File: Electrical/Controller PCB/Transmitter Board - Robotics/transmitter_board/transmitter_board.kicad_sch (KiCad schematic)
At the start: 19 parts, among them SW1 Enable, SW2 Power, SW3 E Stop, U1 AP63203WU, U2 ESP32-S3-ZERO, U3 COM-09032

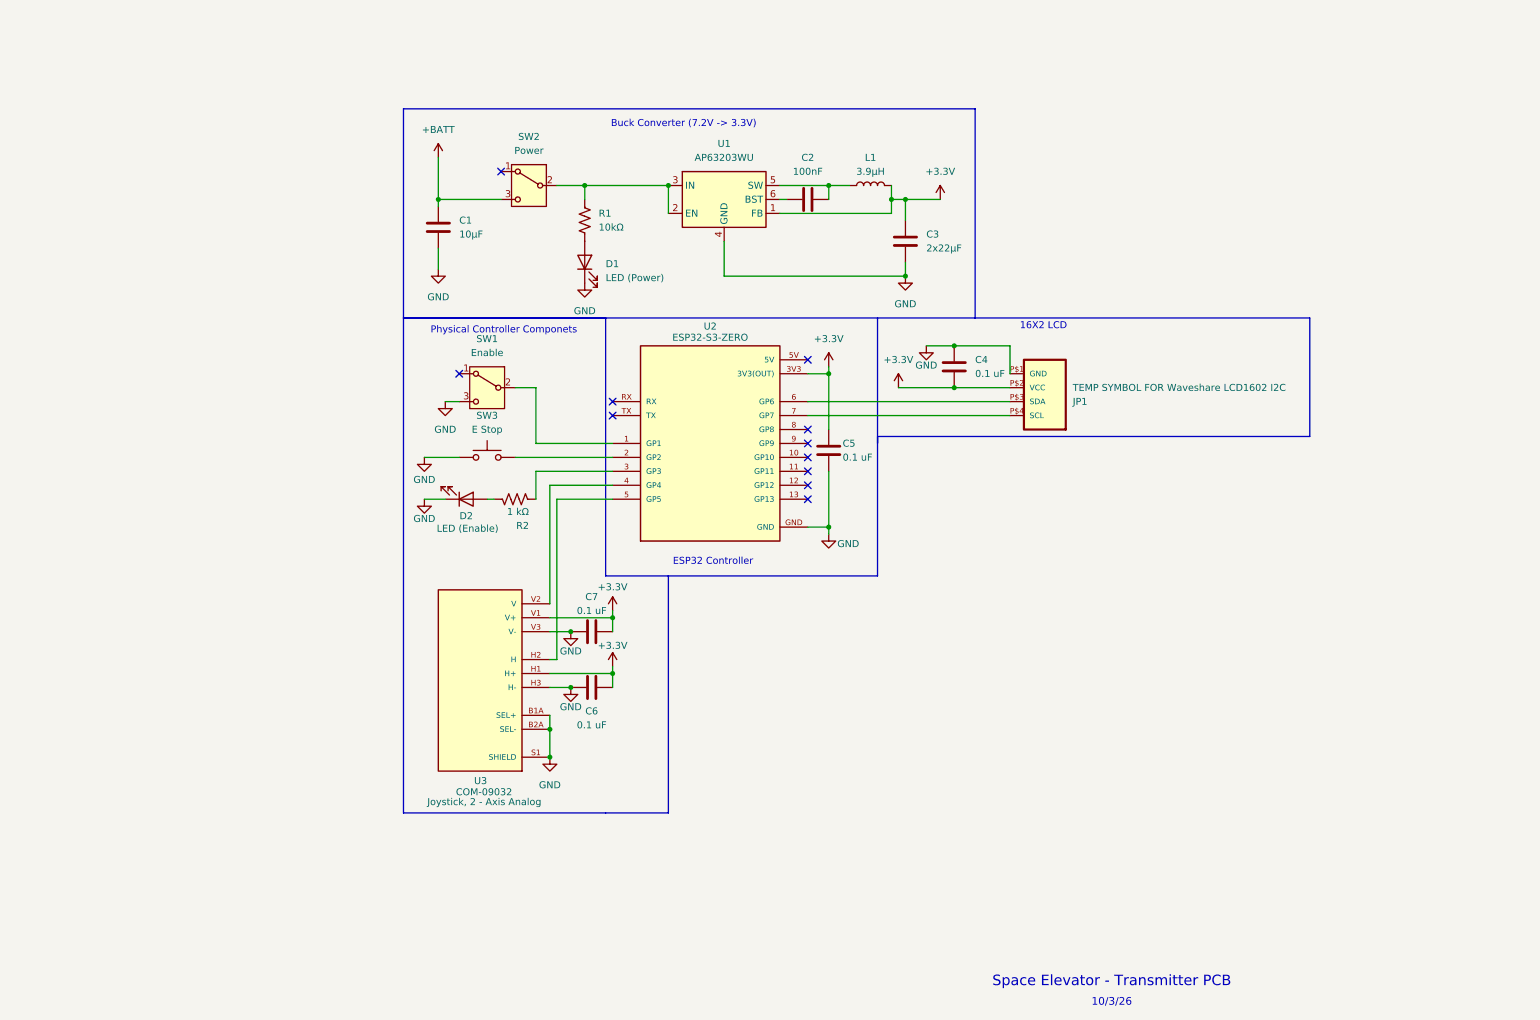
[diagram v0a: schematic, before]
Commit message: Schematic changes to transmitter PCB
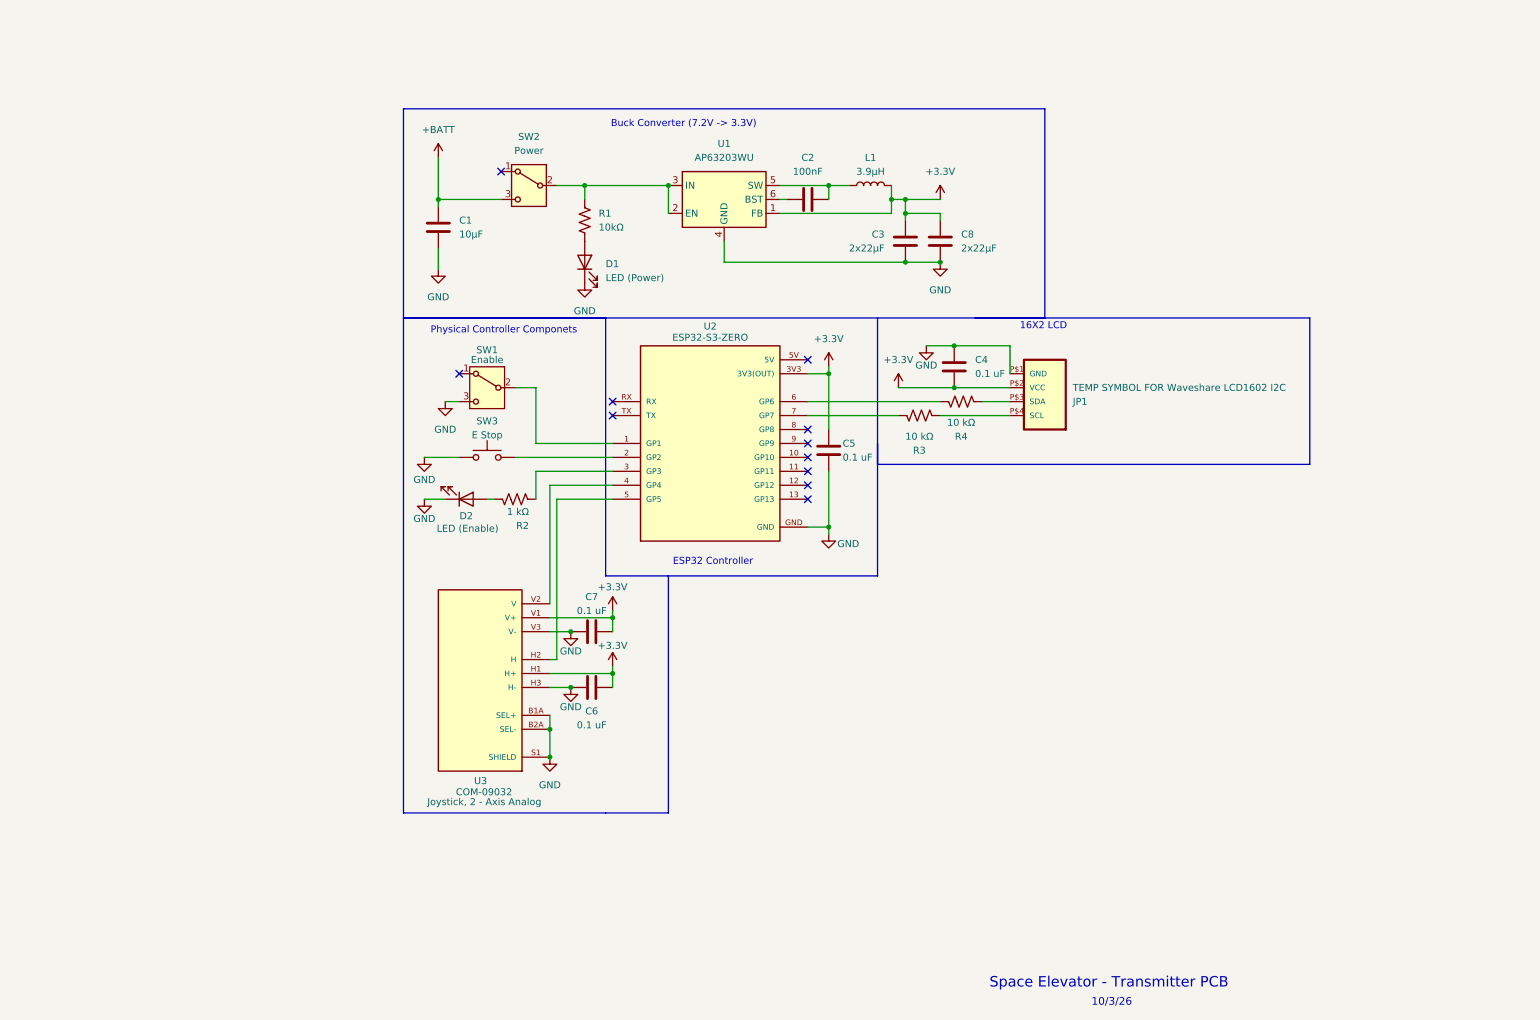
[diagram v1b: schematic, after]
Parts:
- added C8: 2x22µF, symbol Device:C
- added R3, R4: 10 kΩ, PCM_SparkFun-Resistor:R_0603_1608Metric, symbol Device:R_US
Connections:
- net +3.3V: now also C8.1
- net GND: now also C8.2
- net at U2.6 (GP6): now also R4.1; no longer JP1.P$3 (SDA)
- net at U2.7 (GP7): now also R3.1; no longer JP1.P$4 (SCL)
- new net: JP1.P$4 (SCL), R3.2
- new net: JP1.P$3 (SDA), R4.2

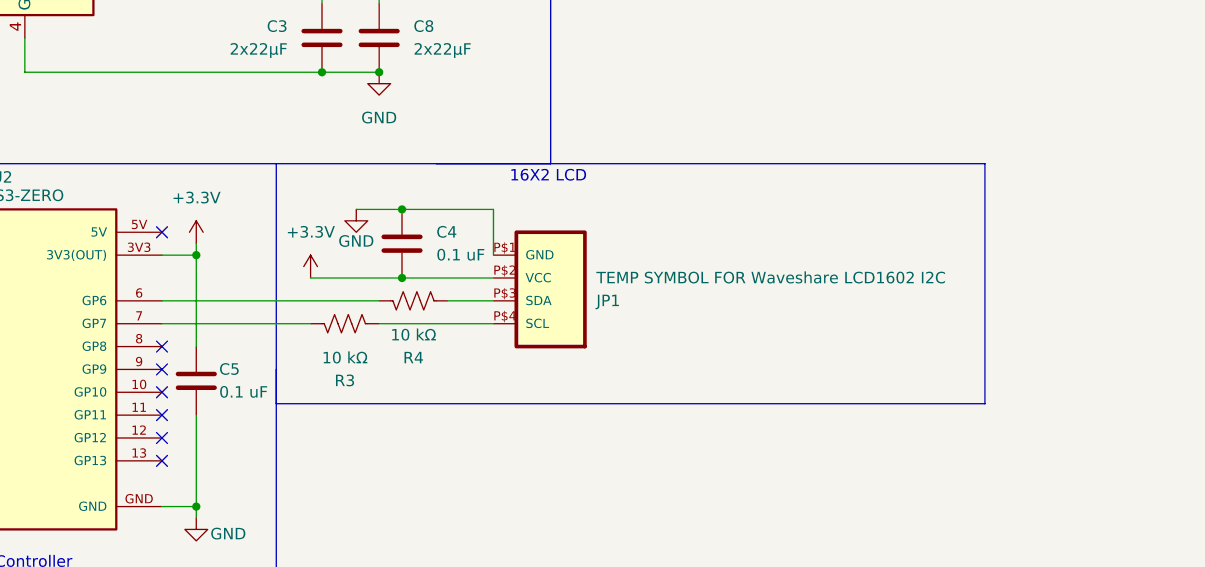
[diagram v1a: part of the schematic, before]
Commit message: Controller PCB updates
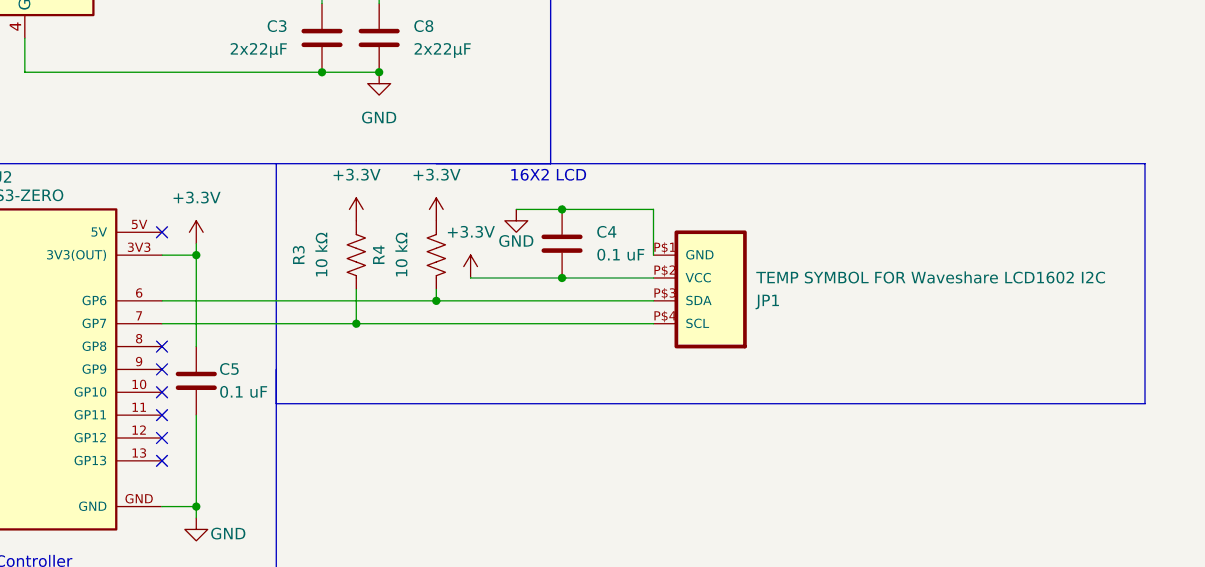
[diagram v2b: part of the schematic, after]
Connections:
- net +3.3V: now also R3.2, R4.1
- net at R3.1, U2.7 (GP7): now also JP1.P$4 (SCL)
- net at U2.6 (GP6): now also JP1.P$3 (SDA), R4.2; no longer R4.1
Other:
- moved on the sheet: C4, JP1, R3, R4

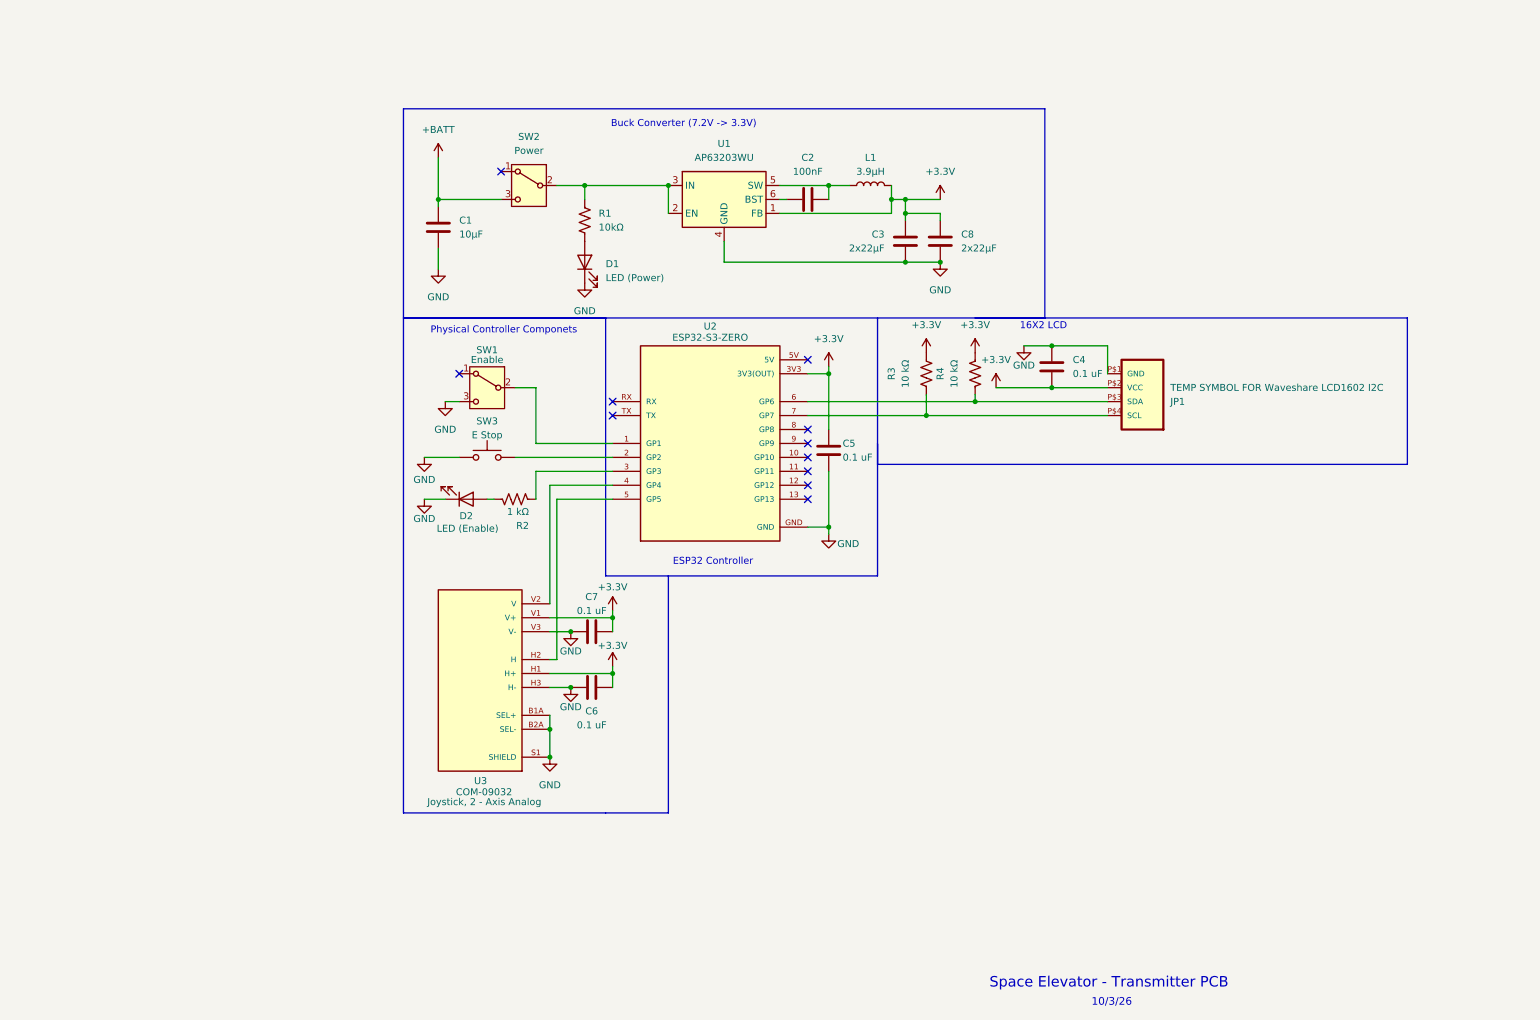
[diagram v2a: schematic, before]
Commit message: Transmitter PCB Schematic updates
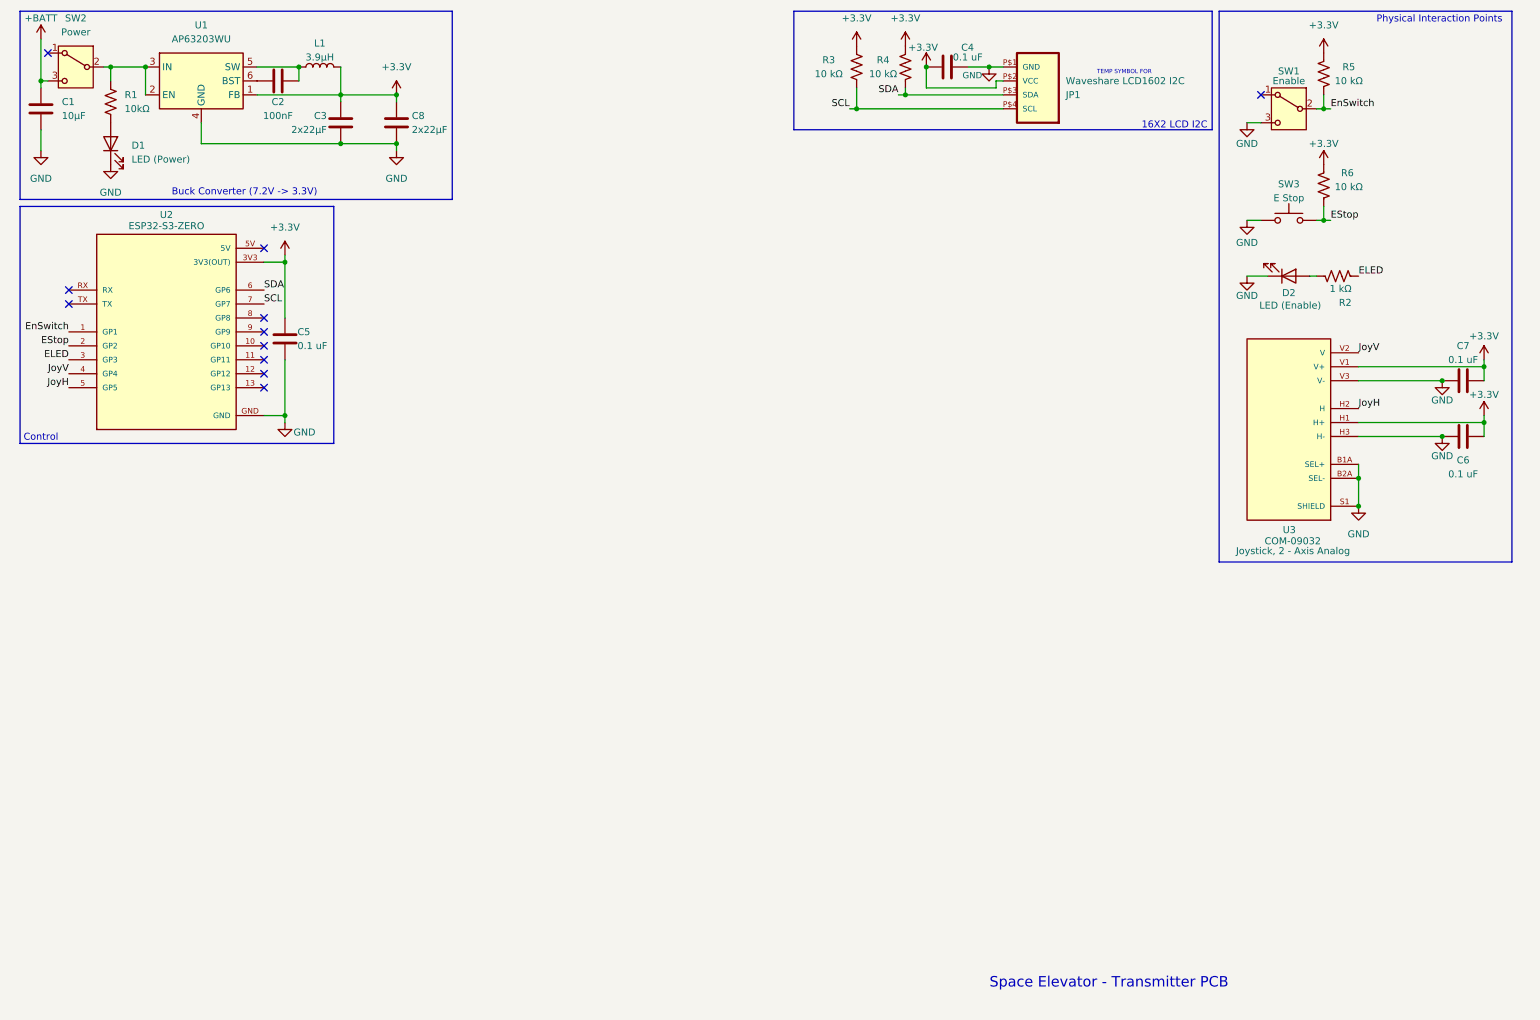
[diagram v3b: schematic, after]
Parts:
- added R5, R6: 10 kΩ, PCM_SparkFun-Resistor:R_0603_1608Metric, symbol Device:R_US
- JP1: value TEMP SYMBOL FOR Waveshare LCD1602 I2C -> Waveshare LCD1602 I2C
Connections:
- net +3.3V: now also C4.1, R5.2, R6.2; no longer C4.2
- net GND: now also C4.2; no longer C4.1
- net SCL: now reaches JP1.P$4 (SCL), R3.1, U2.7 (GP7)
- net EStop: now reaches SW3.2, U2.2 (GP2)
- net EStop: now also R6.1
- net EnSwitch: now reaches SW1.2 (B), U2.1 (GP1)
- net EnSwitch: now also R5.1
- net ELED: now reaches R2.2, U2.3 (GP3)
- net JoyH: now reaches U2.5 (GP5), U3.H2 (H)
- net JoyV: now reaches U2.4 (GP4), U3.V2 (V)
- net SDA: now reaches JP1.P$3 (SDA), R4.2, U2.6 (GP6)
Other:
- note added: "16X2 LCD I2C"
- note added: "Control"
- note added: "Physical Interaction Points"
- note added: "TEMP SYMBOL FOR"
- note removed: "10/3/26"
- note removed: "16X2 LCD"
- note removed: "ESP32 Controller"
- note removed: "Physical Controller Componets"
- moved on the sheet: C1, C2, C3, C4, C5, C6, C7, C8, D1, D2, JP1, L1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

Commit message: Controller PCB updates
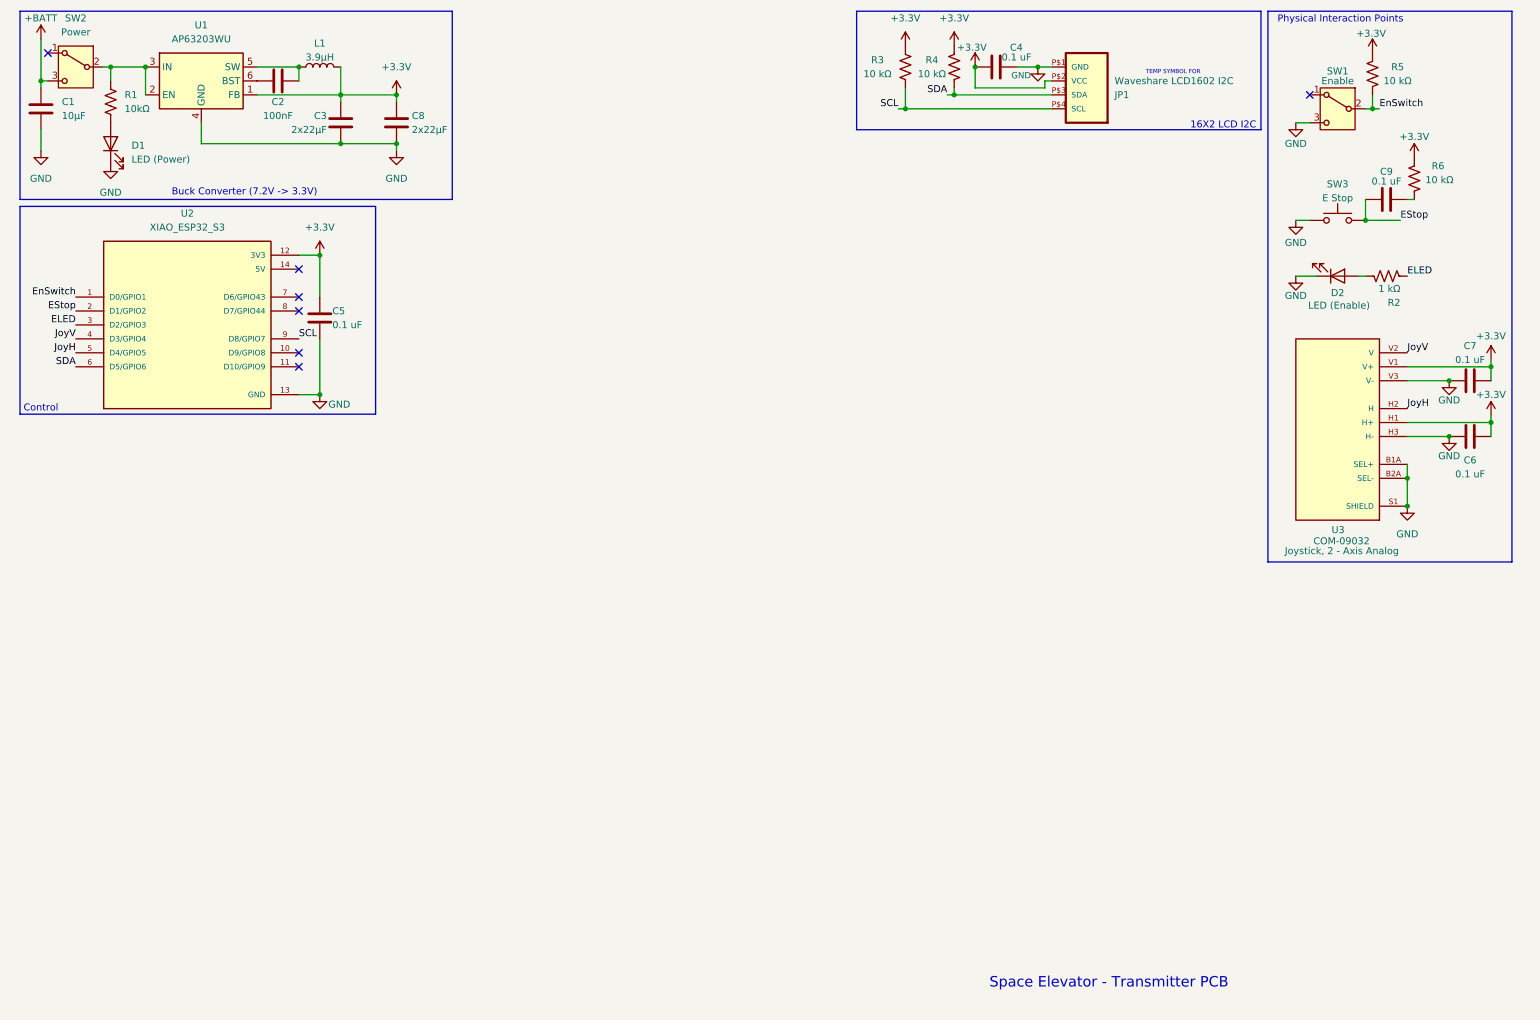
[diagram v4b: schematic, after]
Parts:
- removed U2: ESP32-S3-ZERO, ESP32-S3-ZERO:MODULE_ESP32-S3-ZERO, symbol ESP32-S3-ZERO:ESP32-S3-ZERO
- added C9: 0.1 uF, PCM_SparkFun-Capacitor:C_0603_1608Metric_Polar, symbol Device:C
- added U2: XIAO_ESP32_S3, XIAO_ESP32_S3:MODULE_XIAO_ESP32_S3, symbol XIAO_ESP32_S3:XIAO_ESP32_S3
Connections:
- net +3.3V: now also U2.12 (3V3)
- net ELED: now also U2.3 (D2/GPIO3)
- net EStop: now also C9.1, U2.2 (D1/GPIO2); no longer R6.1
- net EnSwitch: now also U2.1 (D0/GPIO1)
- net GND: now also U2.13 (GND)
- net JoyH: now also U2.5 (D4/GPIO5)
- net JoyV: now also U2.4 (D3/GPIO4)
- net SCL: now also U2.9 (D8/GPIO7)
- net SDA: now also U2.6 (D5/GPIO6)
- new net: C9.2, R6.1
- no-connect marks 11 -> 7
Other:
- moved on the sheet: C4, C6, C7, D2, JP1, R2, R3, R4, R5, R6, SW1, SW3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
